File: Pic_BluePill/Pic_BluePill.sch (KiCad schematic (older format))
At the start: 27 parts, among them J1 Conn_01x14_Male, J2 USB_B_Micro, J3 Conn_01x14_Male, SW1 Swt_btl, SW2 SW_Push, U1 LM78L05, U2 PIC18F2550-ISO, Y1 Crystal

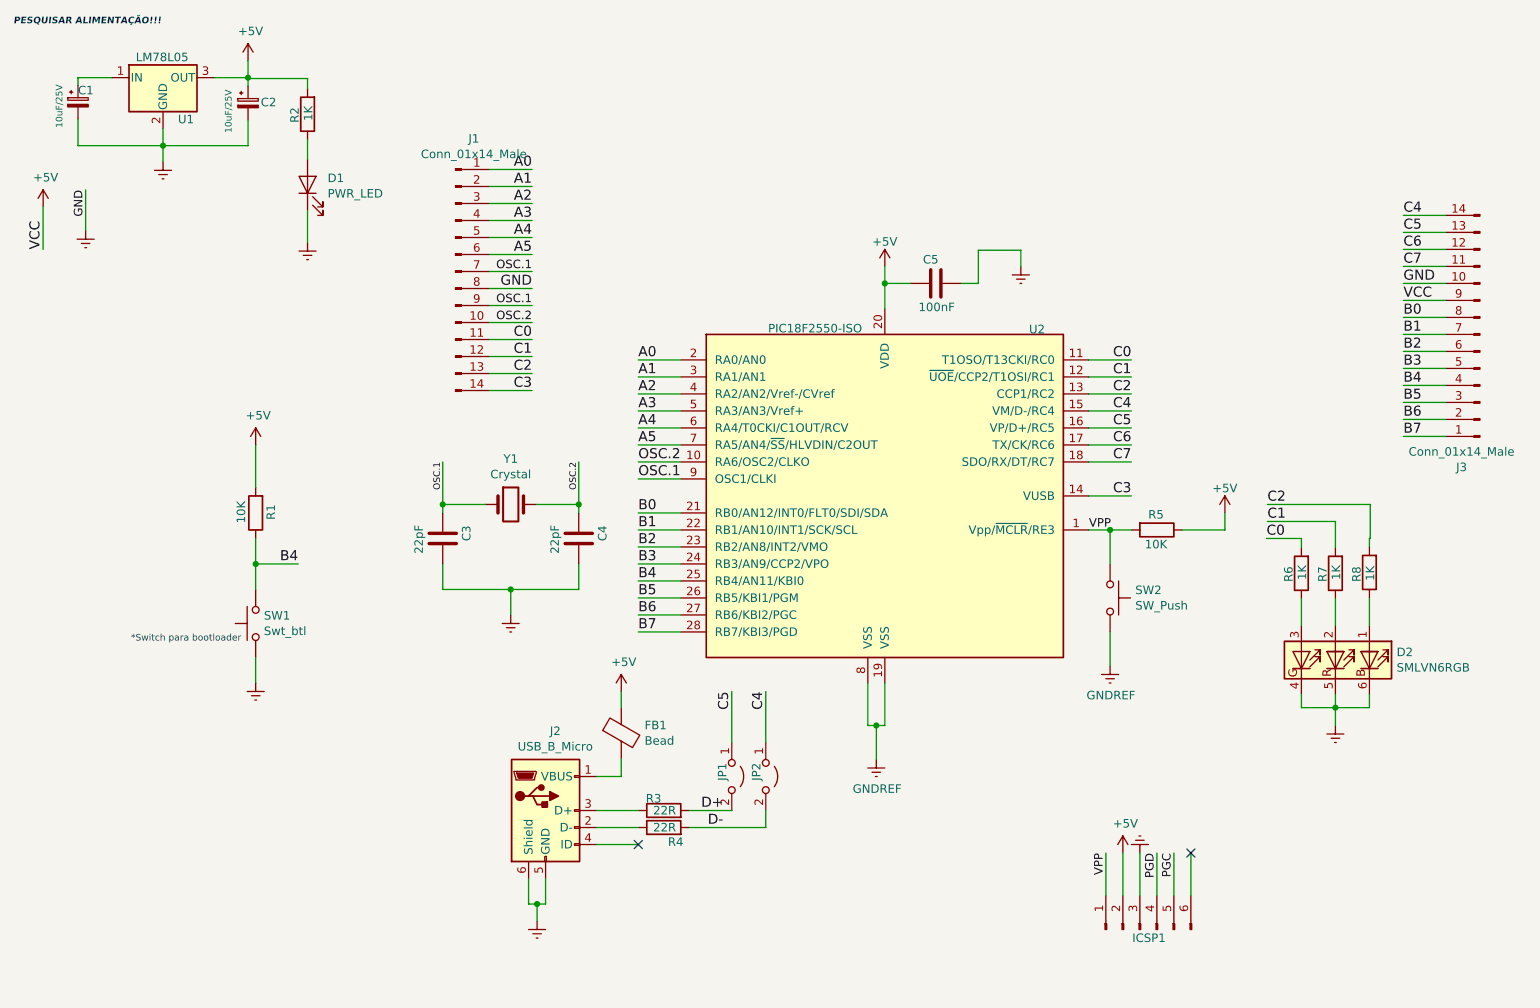
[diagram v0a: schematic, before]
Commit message: Finalização da Placa - sem arquivos de fabricação
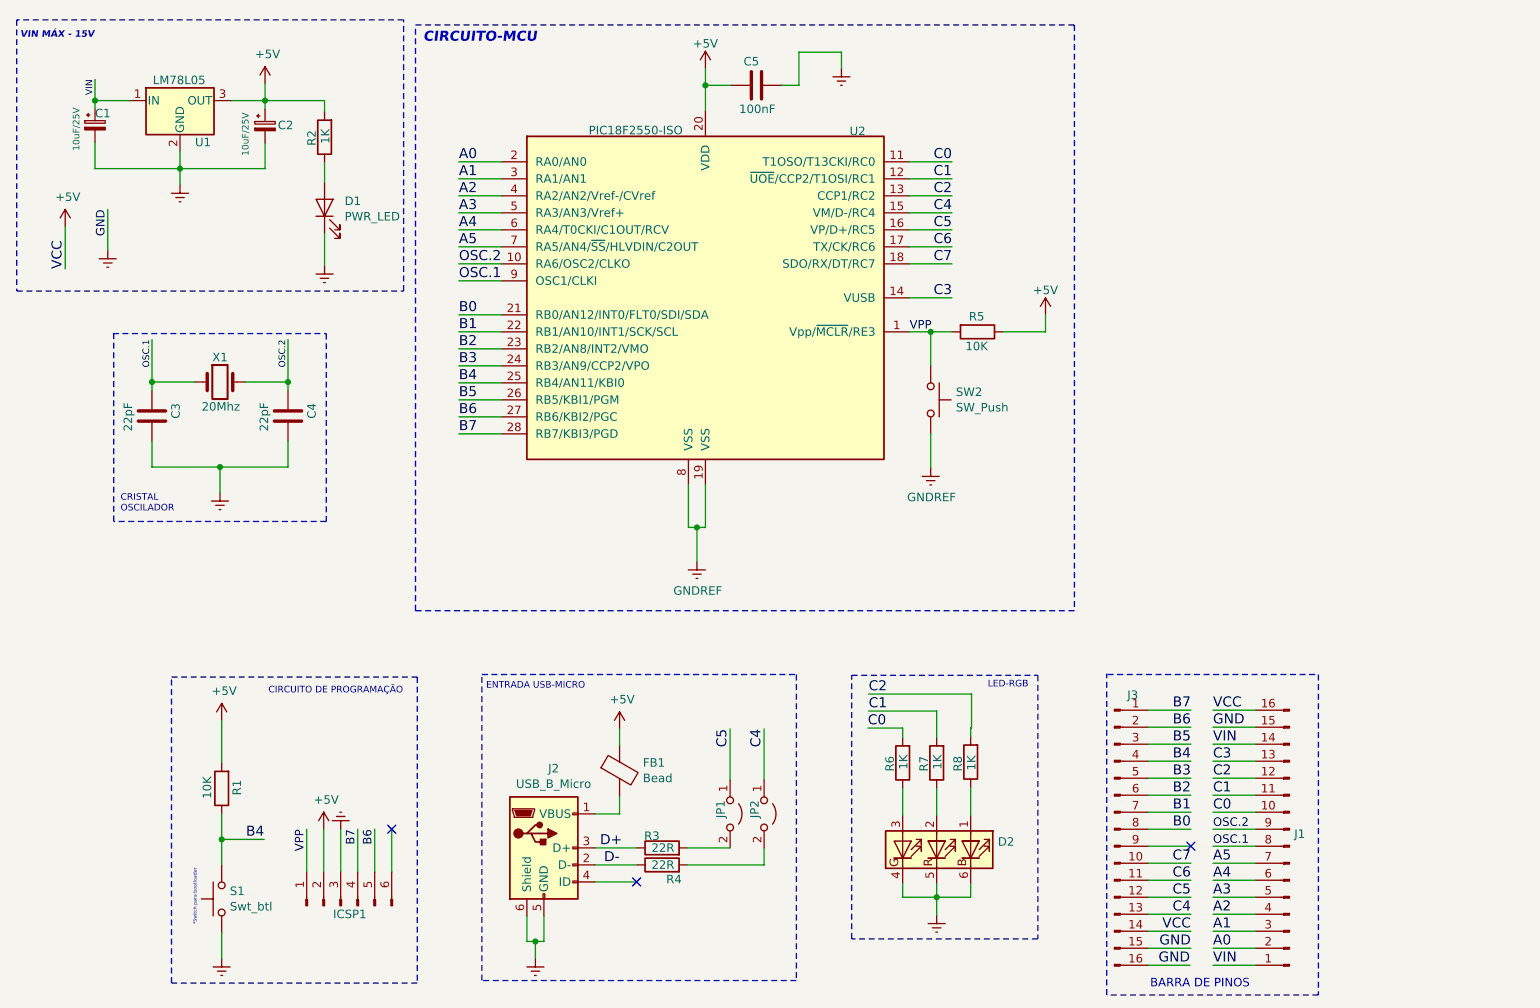
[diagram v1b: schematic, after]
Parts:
- removed J1, J3: Conn_01x14_Male, Connector_PinHeader_2.54mm:PinHeader_1x14_P2.54mm_Vertical, symbol Connector:Conn_01x14_Male
- added J1, J3: Conn_01x16_Male, Connector_PinHeader_2.54mm:PinHeader_1x16_P2.54mm_Vertical, symbol Connector:Conn_01x16_Male
- FB1: footprint (none) -> Capacitor_SMD:C_0805_2012Metric_Pad1.15x1.40mm_HandSolder
- ICSP1: footprint (none) -> Connector_PinHeader_2.54mm:PinHeader_1x06_P2.54mm_Vertical
- JP1, JP2: footprint Connector_PinHeader_2.54mm:PinHeader_1x02_P2.54mm_Vertical -> Jumper:SolderJumper-3_P1.3mm_Open_Pad1.0x1.5mm_NumberLabels
- X1: renamed from Y1; value Crystal -> 20Mhz
- renumbered SW1 to S1
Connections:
- net PGC is gone; now on net B6: ICSP1.5 (Pin_5)
- net PGD is gone; now on net B7: ICSP1.4 (Pin_4)
- net +5V: now also R2.2, J1.16 (Pin_16), J3.14 (Pin_14)
- net A0: now also J1.2 (Pin_2)
- net A1: now also J1.3 (Pin_3)
- net A2: now also J1.4 (Pin_4)
- net A3: now also J1.5 (Pin_5)
- net A4: now also J1.6 (Pin_6)
- net A5: now also J1.7 (Pin_7)
- net B0: now also J3.8 (Pin_8)
- net B1: now also J3.7 (Pin_7)
- net B2: now also J3.6 (Pin_6)
- net B3: now also J3.5 (Pin_5)
- net B4: now also J3.4 (Pin_4)
- net B5: now also J3.3 (Pin_3)
- net B6: now also J3.2 (Pin_2)
- net B7: now also J3.1 (Pin_1)
- net C0: now also J1.10 (Pin_10)
- net C1: now also J1.11 (Pin_11)
- net C2: now also J1.12 (Pin_12)
- net C3: now also J1.13 (Pin_13)
- net C4: now also J3.13 (Pin_13)
- net C5: now also J3.12 (Pin_12)
- net C6: now also J3.11 (Pin_11)
- net C7: now also J3.10 (Pin_10)
- net D+: now also J2.3 (D+), R3.1; no longer JP1.2 (B), R3.2
- net D-: now also J2.2 (D-), R4.1; no longer JP2.2 (B), R4.2
- net GNDREF: now also J1.15 (Pin_15), J3.15 (Pin_15), J3.16 (Pin_16)
- net OSC.1: now also J1.8 (Pin_8)
- net OSC.2: now also J1.9 (Pin_9)
- net VIN: now reaches C1.1, U1.1 (IN)
- net VIN: now also J1.1 (Pin_1), J1.14 (Pin_14)
- new net: JP1.2 (B), R3.2
- new net: JP2.2 (B), R4.2
- no-connect marks 2 -> 3
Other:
- note added: "BARRA DE PINOS\n"
- note added: "CIRCUITO DE PROGRAMAÇÃO\n"
- note added: "CIRCUITO-MCU\n"
- note added: "CRISTAL\nOSCILADOR\n"
- note added: "ENTRADA USB-MICRO\n\n"
- note added: "LED-RGB\n"
- note added: "VIN MÁX - 15V\n\n\n"
- note removed: "PESQUISAR ALIMENTAÇÃO!!!\n"
- moved on the sheet: C1, C2, C3, C4, C5, D1, D2, FB1, ICSP1, J2, JP1, JP2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
